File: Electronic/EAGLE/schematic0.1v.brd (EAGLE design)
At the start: 68.5 x 56.4 mm, 14 parts, among them CN2 1X4SMT, CN3 1X4SMT, J1 JACK2.1MM

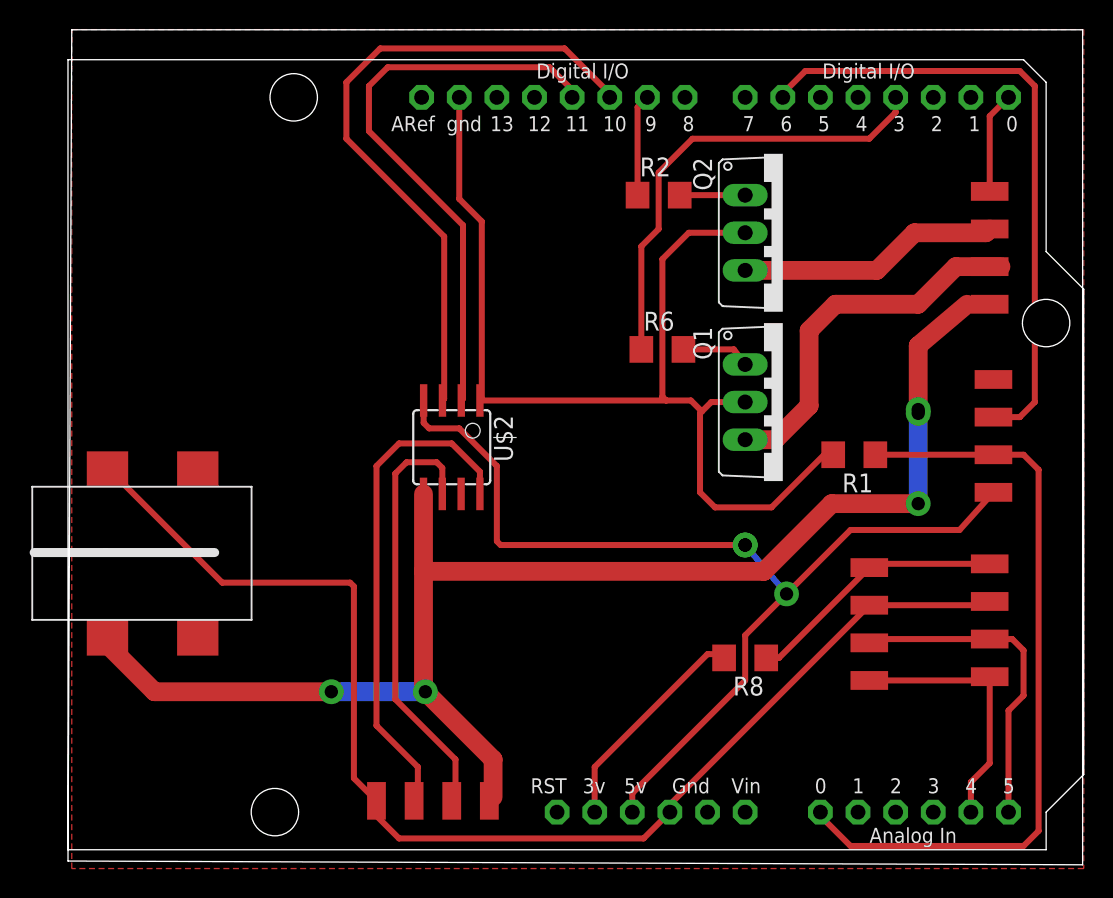
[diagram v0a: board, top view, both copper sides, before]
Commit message: nueva version Pi
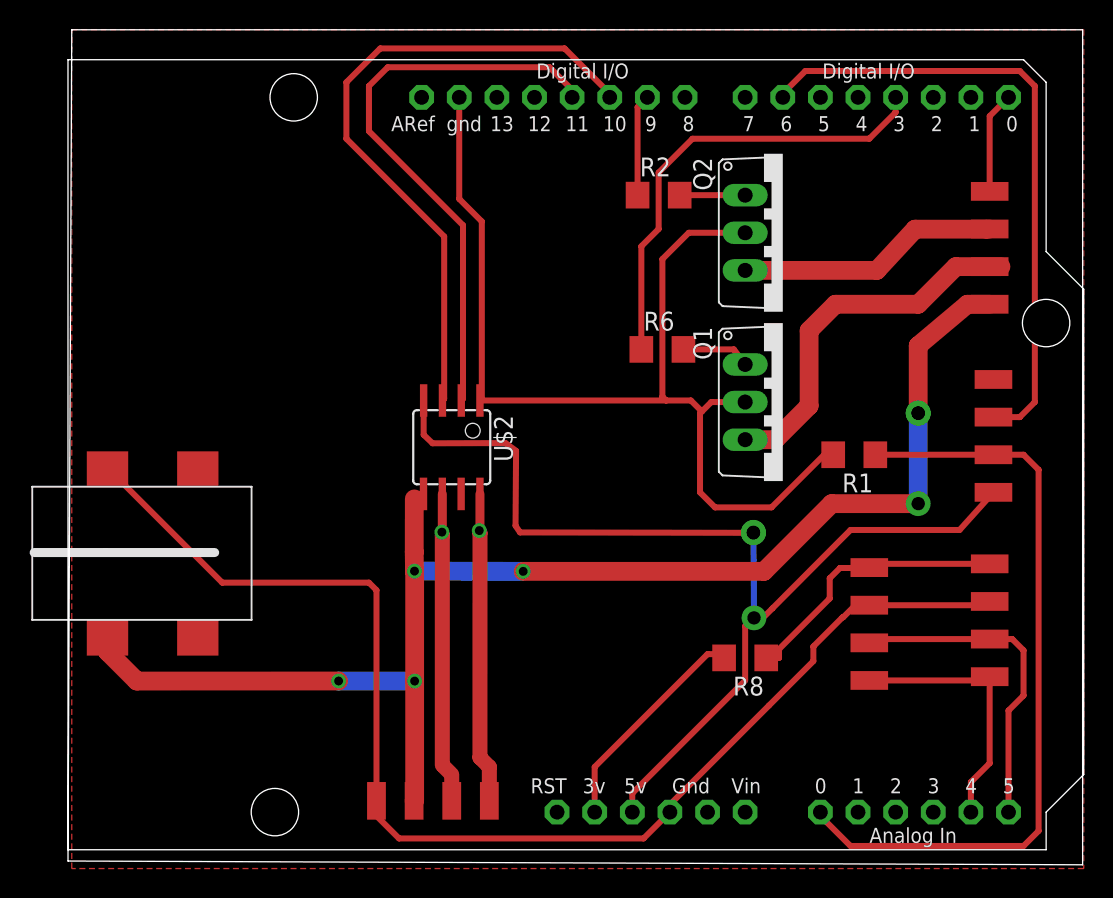
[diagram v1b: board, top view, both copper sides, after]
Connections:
- net PEL_2: now also PELTIER.4; no longer PELTIER.2
- net VCC_12V: now also PELTIER.2; no longer PELTIER.4
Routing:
- net PEL_2: track 33.8 -> 21.0 mm
- net PEL_1: track 29.3 -> 21.0 mm
- net VCC_5V: track 69.9 -> 72.4 mm
- net VCC_12V: track 97.8 -> 96.3 mm, vias 4 -> 6
- net GND1: track 157.0 -> 158.3 mm
- net HT_VCC: track 17.7 -> 18.9 mm
